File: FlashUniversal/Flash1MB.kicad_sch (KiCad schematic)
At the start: 26 parts, among them J1 Conn_02x04_Odd_Even, J10 Conn_01x01_Pin, J11 Conn_01x01_Pin, J12 Conn_01x01_Pin, J13 Conn_01x01_Pin, J14 Conn_01x01_Pin, J15 Conn_01x01_Pin, J16 Conn_01x01_Pin, J17 Conn_01x01_Pin, J18 Conn_01x01_Pin, J19 Conn_01x01_Pin, J2 Conn_01x01_Pin, J20 Conn_01x01_Pin, J21 Conn_01x01_Pin, J22 Conn_01x01_Pin, J3 Conn_01x01_Pin, J4 Conn_01x01_Pin, J5 Conn_01x01_Pin, J6 Conn_01x01_Pin, J7 Conn_01x01_Pin, J8 Conn_01x01_Pin, J9 Conn_01x01_Pin

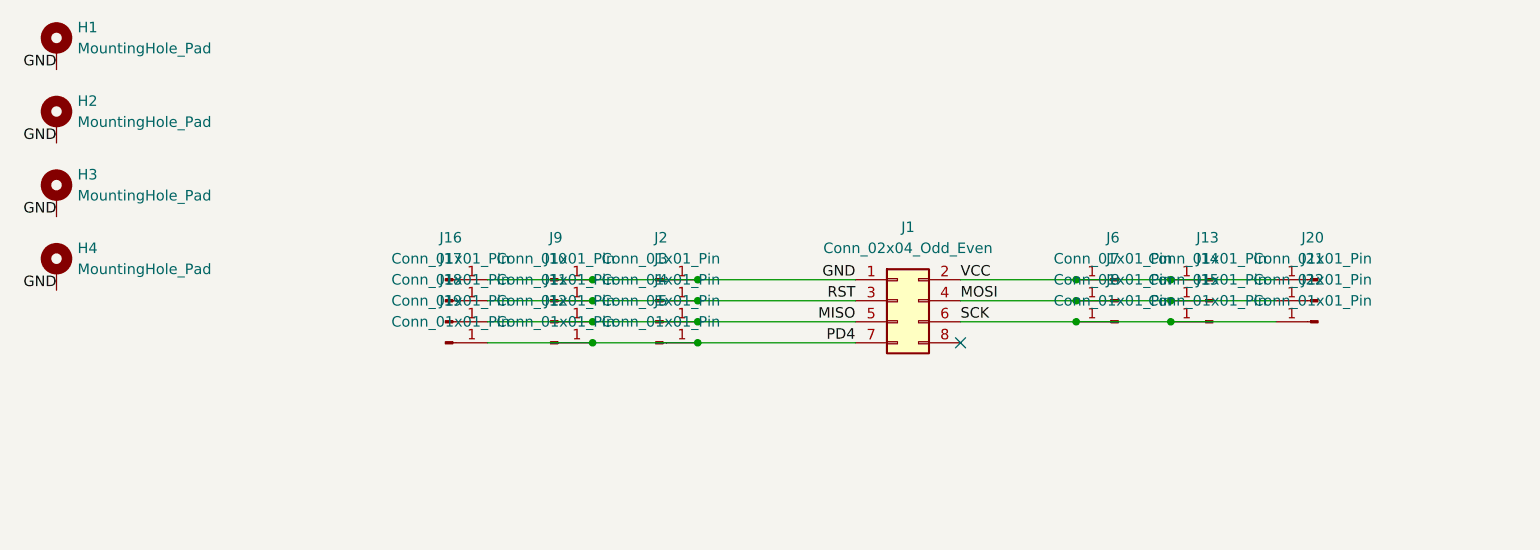
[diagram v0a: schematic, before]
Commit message: kicad 9 update
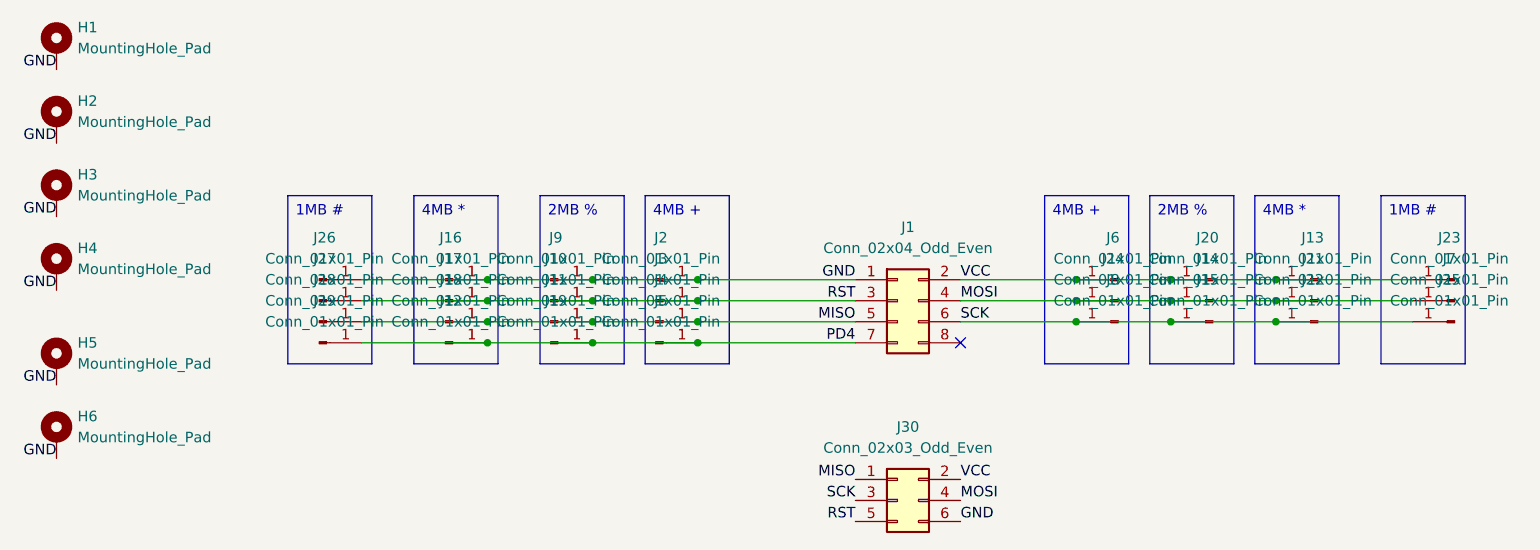
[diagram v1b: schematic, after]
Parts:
- added H5, H6: MountingHole_Pad, MountingHole:MountingHole_2.2mm_M2_DIN965_Pad, symbol Mechanical:MountingHole_Pad
- added J23, J24, J25, J26, J27, J28, J29: Conn_01x01_Pin, Connector_PinHeader_2.54mm:PinHeader_1x01_P2.54mm_Vertical, symbol Connector:Conn_01x01_Pin
- added J30: Conn_02x03_Odd_Even, Connector_PinHeader_2.54mm:PinHeader_2x03_P2.54mm_Vertical, symbol Connector_Generic:Conn_02x03_Odd_Even
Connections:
- net GND: now also H5.1, H6.1, J26.1 (Pin_1), J30.6 (Pin_6)
- net MISO: now also J28.1 (Pin_1), J30.1 (Pin_1)
- net MOSI: now also J24.1 (Pin_1), J30.4 (Pin_4)
- net PD4: now also J29.1 (Pin_1)
- net RST: now also J27.1 (Pin_1), J30.5 (Pin_5)
- net SCK: now also J25.1 (Pin_1), J30.3 (Pin_3)
- net VCC: now also J23.1 (Pin_1), J30.2 (Pin_2)
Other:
- moved on the sheet: J12, J13, J19, J20, J7

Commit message: loch
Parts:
- H1, H2, H3, H4: footprint MountingHole:MountingHole_4mm_Pad -> MountingHole:MountingHole_4.3mm_M4_DIN965_Pad
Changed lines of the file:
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@@
 			)
 		)
-		(property "Footprint" "MountingHole:MountingHole_4mm_Pad"
+		(property "Footprint" "MountingHole:MountingHole_4.3mm_M4_DIN965_Pad"
 			(at 20.32 49.53 0)
 			(effects
@@
 			)
 		)
-		(property "Footprint" "MountingHole:MountingHole_4mm_Pad"
+		(property "Footprint" "MountingHole:MountingHole_4.3mm_M4_DIN965_Pad"
 			(at 20.32 31.75 0)
 			(effects
@@
 			)
 		)
-		(property "Footprint" "MountingHole:MountingHole_4mm_Pad"
+		(property "Footprint" "MountingHole:MountingHole_4.3mm_M4_DIN965_Pad"
 			(at 20.32 40.64 0)
 			(effects
@@
 			)
 		)
-		(property "Footprint" "MountingHole:MountingHole_4mm_Pad"
+		(property "Footprint" "MountingHole:MountingHole_4.3mm_M4_DIN965_Pad"
 			(at 20.32 22.86 0)
 			(effects
